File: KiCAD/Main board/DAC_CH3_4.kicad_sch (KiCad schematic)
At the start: 51 parts, among them U1 PCM1789-Q1, U3 OPA1632DR, U4 OPA1632DR

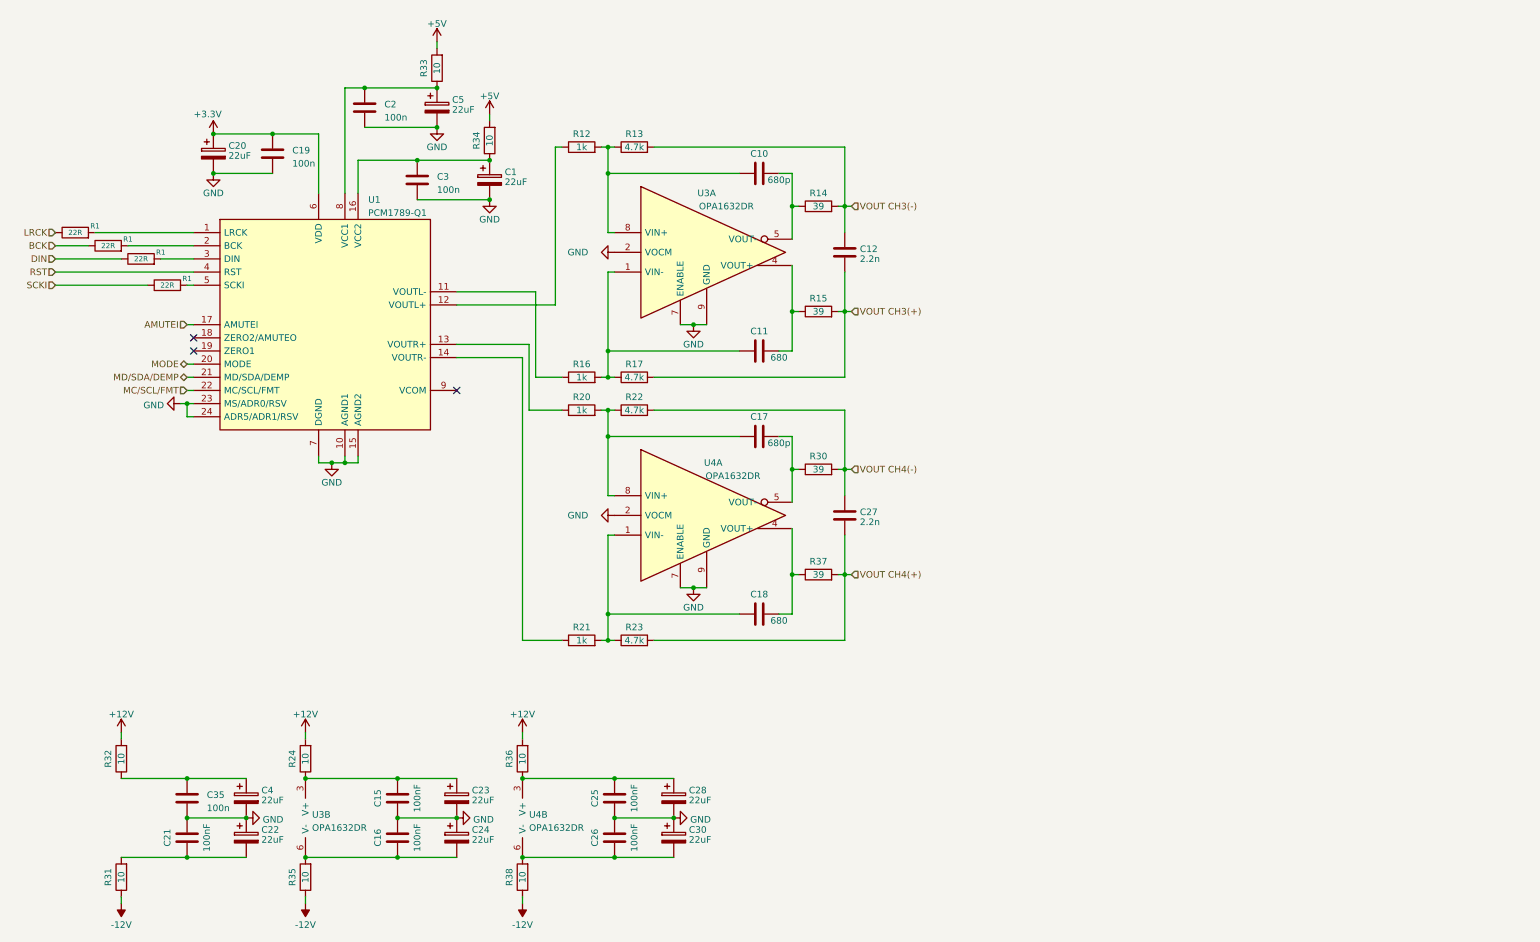
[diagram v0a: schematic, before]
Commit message: Worked a bit on the main board
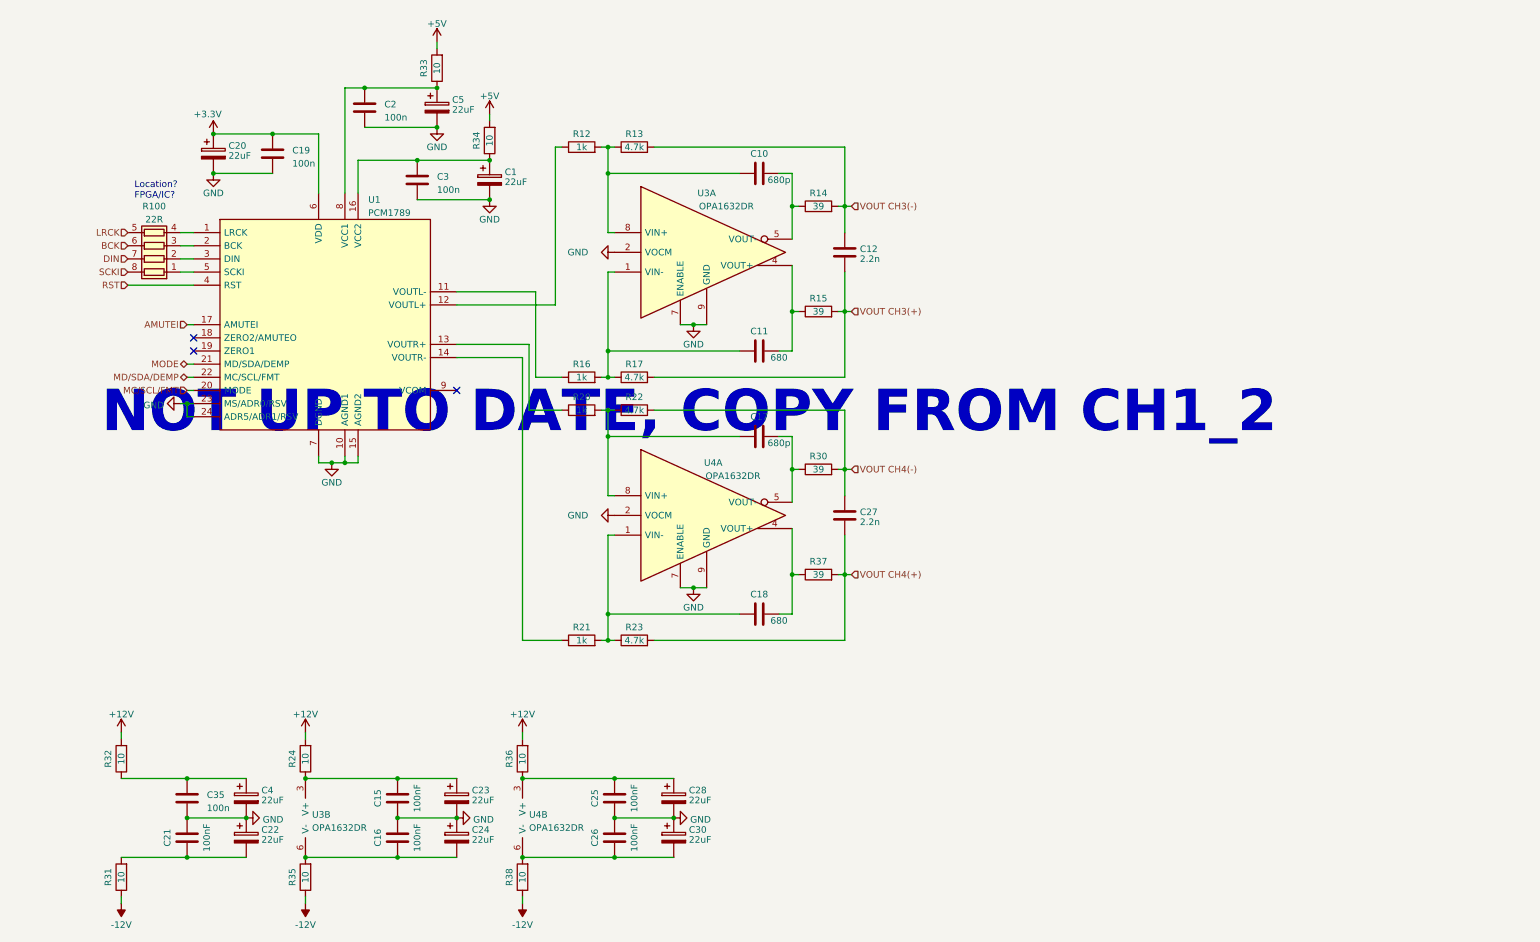
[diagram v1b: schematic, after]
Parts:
- removed R1 (x4): 22R, Resistor_SMD:R_0805_2012Metric, symbol Device:R
- removed U1: PCM1789-Q1, Package_SO:TSSOP-24_4.4x7.8mm_P0.65mm, symbol Audio-DSP:PCM1789-Q1
- added R100: 22R, Resistor_SMD:R_Array_Convex_4x0402, symbol Device:R_Pack04
- added U1: PCM1789, Package_SO:TSSOP-24_4.4x7.8mm_P0.65mm, symbol Audio-DSP:PCM1789
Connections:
- net +3.3V: now also U1.6 (VDD)
- net AMUTEI: now also U1.17 (AMUTEI)
- net BCK: now also R100.6 (R3.2)
- net DIN: now also R100.7 (R2.2)
- net GND: now also U1.10 (AGND1), U1.15 (AGND2), U1.23 (MS/ADR0/RSV), U1.24 (ADR5/ADR1/RSV), U1.7 (DGND)
- net LRCK: now also R100.5 (R4.2)
- net MC/SCL/FMT: now also U1.20 (MODE)
- net MD/SDA/DEMP: now also U1.22 (MC/SCL/FMT)
- net MODE: now also U1.21 (MD/SDA/DEMP)
- net RST: now also U1.4 (RST)
- net SCKI: now also R100.8 (R1.2)
- net at R20.1: now also U1.13 (VOUTR+)
- net at C2.1, C5.1, R33.1: now also U1.8 (VCC1)
- net at R12.1: now also U1.12 (VOUTL+)
- net at R21.1: now also U1.14 (VOUTR-)
- net at R16.1: now also U1.11 (VOUTL-)
- net at C1.1, C3.1, R34.1: now also U1.16 (VCC2)
- new net: R100.4 (R4.1), U1.1 (LRCK)
- new net: R100.3 (R3.1), U1.2 (BCK)
- new net: R100.2 (R2.1), U1.3 (DIN)
- new net: R100.1 (R1.1), U1.5 (SCKI)
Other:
- note added: "Location? FPGA/IC?"
- note added: "NOT UP TO DATE, COPY FROM CH1_2"

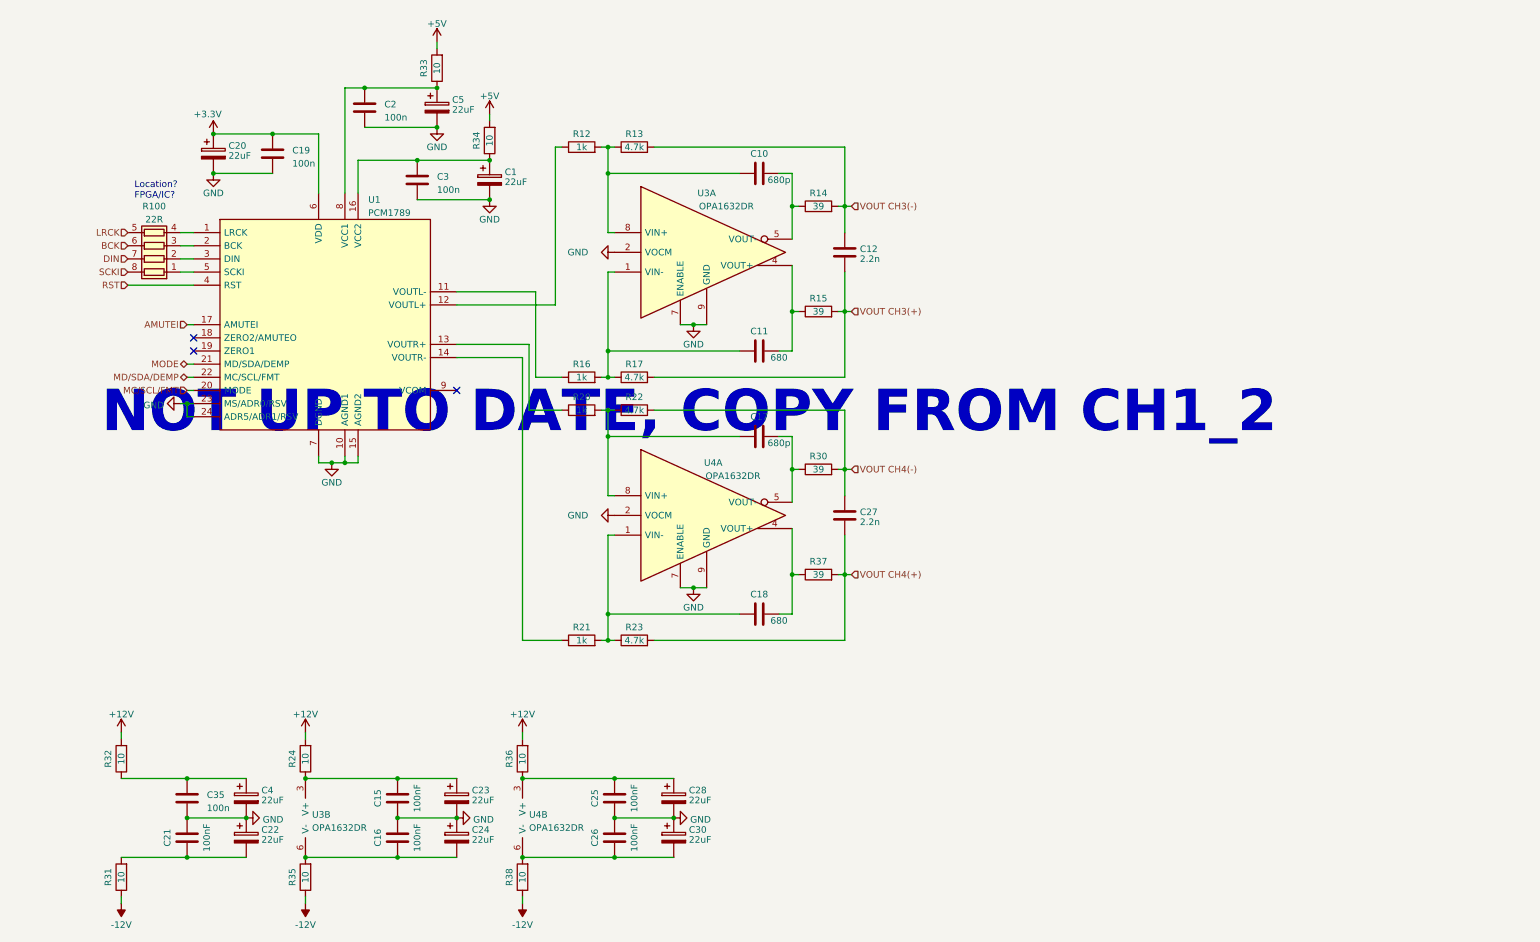
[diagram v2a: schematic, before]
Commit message: Worked on main board
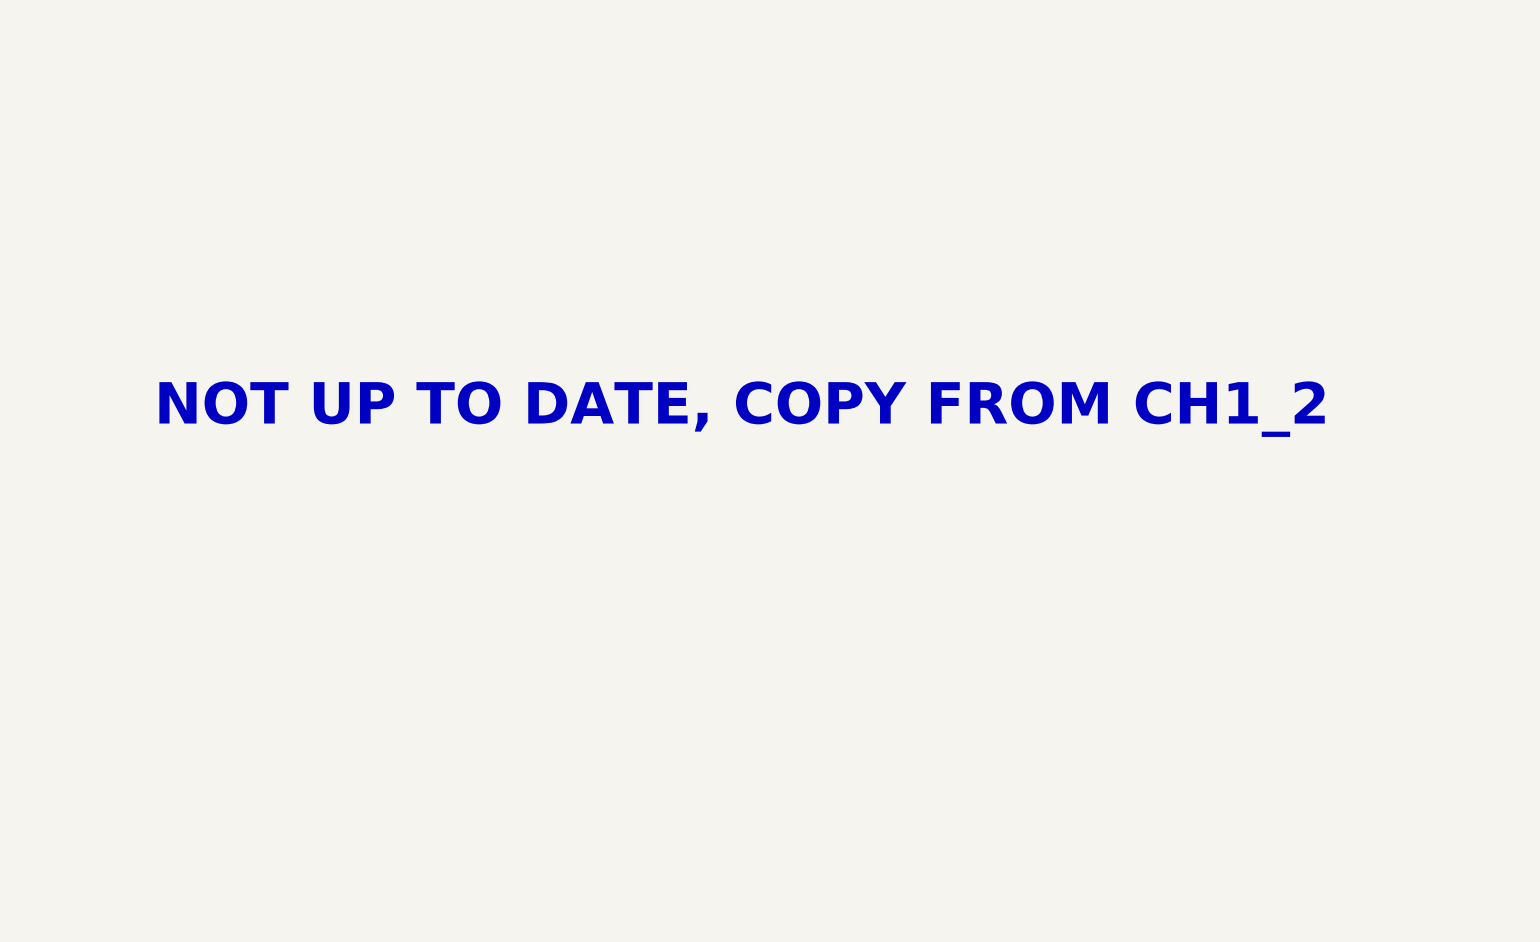
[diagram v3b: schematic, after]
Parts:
- removed C1, C20, C22, C23, C24, C28, C30, C4, C5: 22uF, Capacitor_THT:CP_Radial_D5.0mm_P2.00mm, symbol Device:C_Polarized
- removed C10, C17: 680p, Capacitor_SMD:C_0805_2012Metric, symbol Device:C
- removed C11, C18: 680, Capacitor_SMD:C_0805_2012Metric, symbol Device:C
- removed C12, C27: 2.2n, Capacitor_SMD:C_0805_2012Metric, symbol Device:C
- removed C15, C16, C21, C25, C26: 100nF, Capacitor_SMD:C_0805_2012Metric, symbol Device:C
- removed C19, C2, C3, C35: 100n, Capacitor_SMD:C_0805_2012Metric, symbol Device:C
- removed R100: 22R, Resistor_SMD:R_Array_Convex_4x0402, symbol Device:R_Pack04
- removed R12, R16, R20, R21: 1k, Resistor_SMD:R_0805_2012Metric, symbol Device:R
- removed R13, R17, R22, R23: 4.7k, Resistor_SMD:R_0805_2012Metric, symbol Device:R
- removed R14, R15, R30, R37: 39, Resistor_SMD:R_0805_2012Metric, symbol Device:R
- removed R24, R31, R32, R33, R34, R35, R36, R38: 10, Resistor_SMD:R_0805_2012Metric, symbol Device:R
- removed U1: PCM1789, Package_SO:TSSOP-24_4.4x7.8mm_P0.65mm, symbol Audio-DSP:PCM1789
- removed U3, U4: OPA1632DR, Audio_DSP:VSSOP-8_3.0x3.0mm_P0.65_TP1.8x1.5, symbol Audio-DSP:OPA1632DR
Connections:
- no-connect marks 3 -> 0
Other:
- note removed: "Location? FPGA/IC?"

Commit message: Worked on SDD, main board schematic and LTspice discrete linear regulator
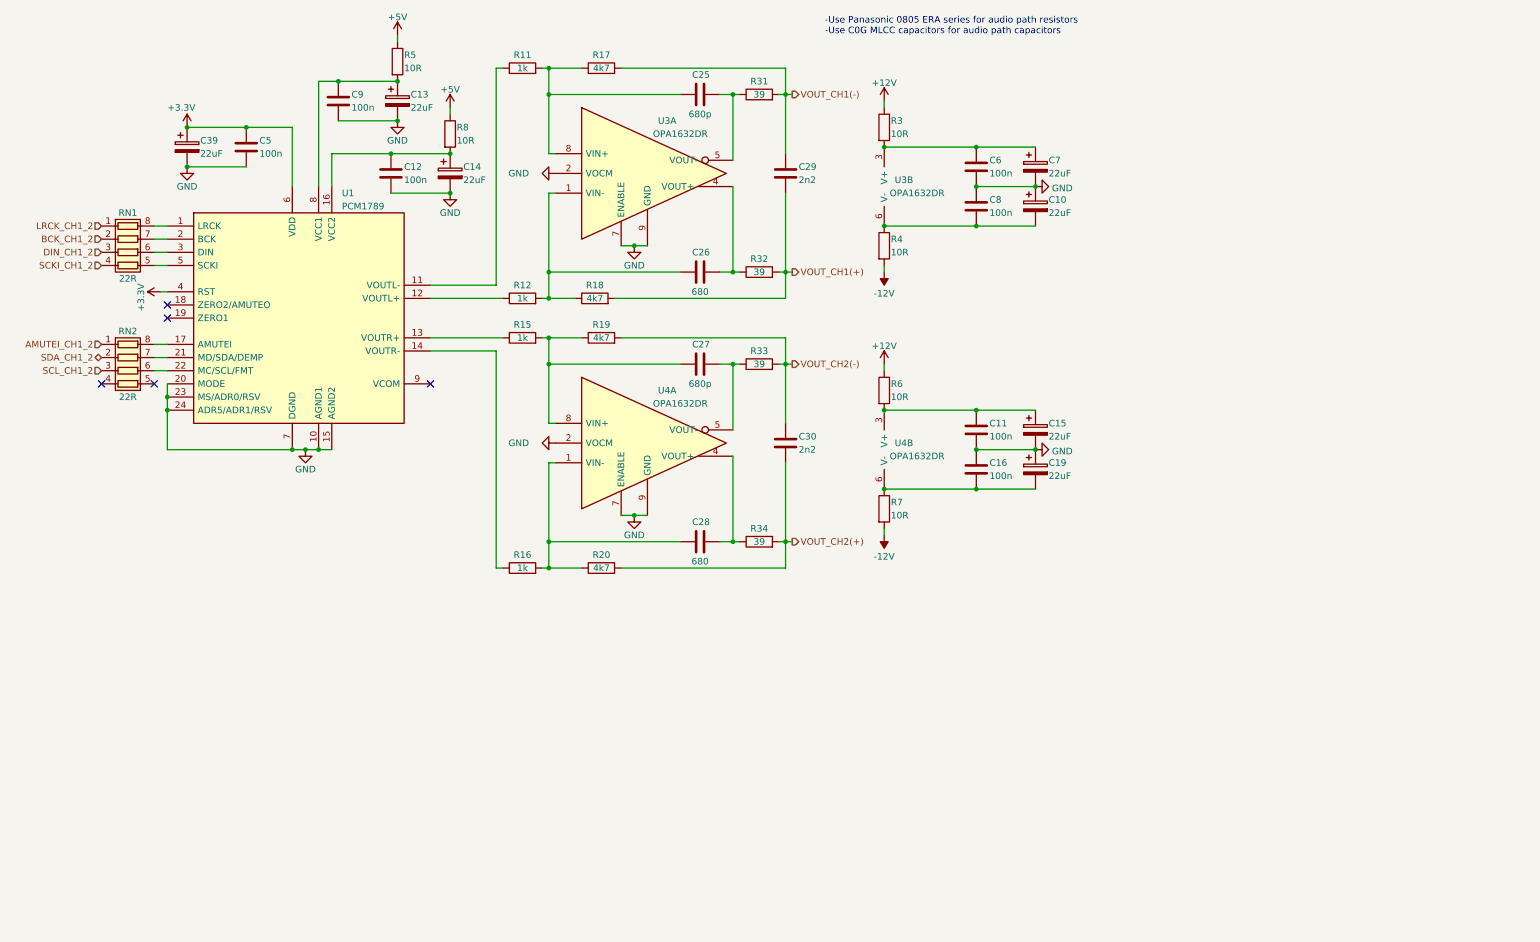
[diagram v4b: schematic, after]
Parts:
- added C10, C13, C14, C15, C19, C39, C7: 22uF, Capacitor_THT:CP_Radial_D5.0mm_P2.00mm, symbol Device:C_Polarized
- added C11, C12, C16, C5, C6, C8, C9: 100n, Capacitor_SMD:C_0402_1005Metric, symbol Device:C
- added C25, C27: 680p, Capacitor_SMD:C_0805_2012Metric, symbol Device:C
- added C26, C28: 680, Capacitor_SMD:C_0805_2012Metric, symbol Device:C
- added C29, C30: 2n2, Capacitor_SMD:C_0805_2012Metric, symbol Device:C
- added R11, R12, R15, R16: 1k, Resistor_SMD:R_0805_2012Metric, symbol Device:R
- added R17, R18, R19, R20: 4k7, Resistor_SMD:R_0805_2012Metric, symbol Device:R
- added R3, R4, R5, R6, R7, R8: 10R, Resistor_SMD:R_0805_2012Metric, symbol Device:R
- added R31, R32, R33, R34: 39, Resistor_SMD:R_0805_2012Metric, symbol Device:R
- added RN1, RN2: 22R, Resistor_SMD:R_Array_Convex_4x0402, symbol Device:R_Pack04
- added U1: PCM1789, Package_SO:TSSOP-24_4.4x7.8mm_P0.65mm, symbol Audio_DSP:PCM1789
- added U3, U4: OPA1632DR, Audio-DSP:VSSOP-8_3.0x3.0mm_P0.65_TP1.8x1.5, symbol Audio-DSP:OPA1632DR
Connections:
- new net: C6.1, C7.1, R3.2, U3.3 (V+)
- new net: C26.1, R12.2, R18.1, U3.1 (VIN-)
- new net: C26.2, R32.1, U3.4 (VOUT+)
- new net: C25.2, R31.1, U3.5 (VOUT-)
- new net: C25.1, R11.2, R17.1, U3.8 (VIN+)
- new net: C28.1, R16.2, R20.1, U4.1 (VIN-)
- new net: C12.1, C14.1, R8.2, U1.16 (VCC2)
- new net: C10.2, C8.2, R4.1, U3.6 (V-)
- new net: C28.2, R34.1, U4.4 (VOUT+)
- new net: C16.2, C19.2, R7.1, U4.6 (V-)
- new net: RN2.6 (R3.2), U1.22 (MC/SCL/FMT)
- new net: RN2.7 (R2.2), U1.21 (MD/SDA/DEMP)
- new net: RN2.8 (R1.2), U1.17 (AMUTEI)
- new net: C27.2, R33.1, U4.5 (VOUT-)
- new net: C27.1, R15.2, R19.1, U4.8 (VIN+)
- new net: R11.1, U1.11 (VOUTL-)
- new net: C11.1, C15.1, R6.2, U4.3 (V+)
- new net: RN1.5 (R4.2), U1.5 (SCKI)
- new net: RN1.6 (R3.2), U1.3 (DIN)
- new net: RN1.7 (R2.2), U1.2 (BCK)
- new net: RN1.8 (R1.2), U1.1 (LRCK)
- new net: R15.1, U1.13 (VOUTR+)
- new net: C13.1, C9.1, R5.2, U1.8 (VCC1)
- new net: R12.1, U1.12 (VOUTL+)
- new net: R16.1, U1.14 (VOUTR-)
- new net +12V: R3.1, R6.1
- new net +3.3V: C39.1, C5.1, U1.4 (RST), U1.6 (VDD)
- new net +5V: R5.1, R8.1
- new net -12V: R4.2, R7.2
- new net AMUTEI_CH1_2: RN2.1 (R1.1)
- new net BCK_CH1_2: RN1.2 (R2.1)
- new net DIN_CH1_2: RN1.3 (R3.1)
- new net GND: C10.1, C11.2, C12.2, C13.2, C14.2, C15.2, C16.1, C19.1, C39.2, C5.2, C6.2, C7.2, C8.1, C9.2, U1.10 (AGND1), U1.15 (AGND2), U1.20 (MODE), U1.23 (MS/ADR0/RSV), U1.24 (ADR5/ADR1/RSV), U1.7 (DGND), U3.2 (VOCM), U3.7 (ENABLE), U3.9 (GND), U4.2 (VOCM), U4.7 (ENABLE), U4.9 (GND)
- new net LRCK_CH1_2: RN1.1 (R1.1)
- new net SCKI_CH1_2: RN1.4 (R4.1)
- new net SCL_CH1_2: RN2.3 (R3.1)
- new net SDA_CH1_2: RN2.2 (R2.1)
- new net VOUT_CH1(+): C29.2, R18.2, R32.2
- new net VOUT_CH1(-): C29.1, R17.2, R31.2
- new net VOUT_CH2(+): C30.2, R20.2, R34.2
- new net VOUT_CH2(-): C30.1, R19.2, R33.2
- no-connect marks 0 -> 5
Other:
- note added: "-Use Panasonic 0805 ERA series for audio path resistors -Use C0G MLCC capacitors for audio path capacitors"
- note removed: "NOT UP TO DATE, COPY FROM CH1_2"
